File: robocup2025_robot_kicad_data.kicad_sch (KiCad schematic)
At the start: 3 parts, among them U2 ESP32-DEVKITC-32E, U4 RASPBERRY_PI_4B_4GB

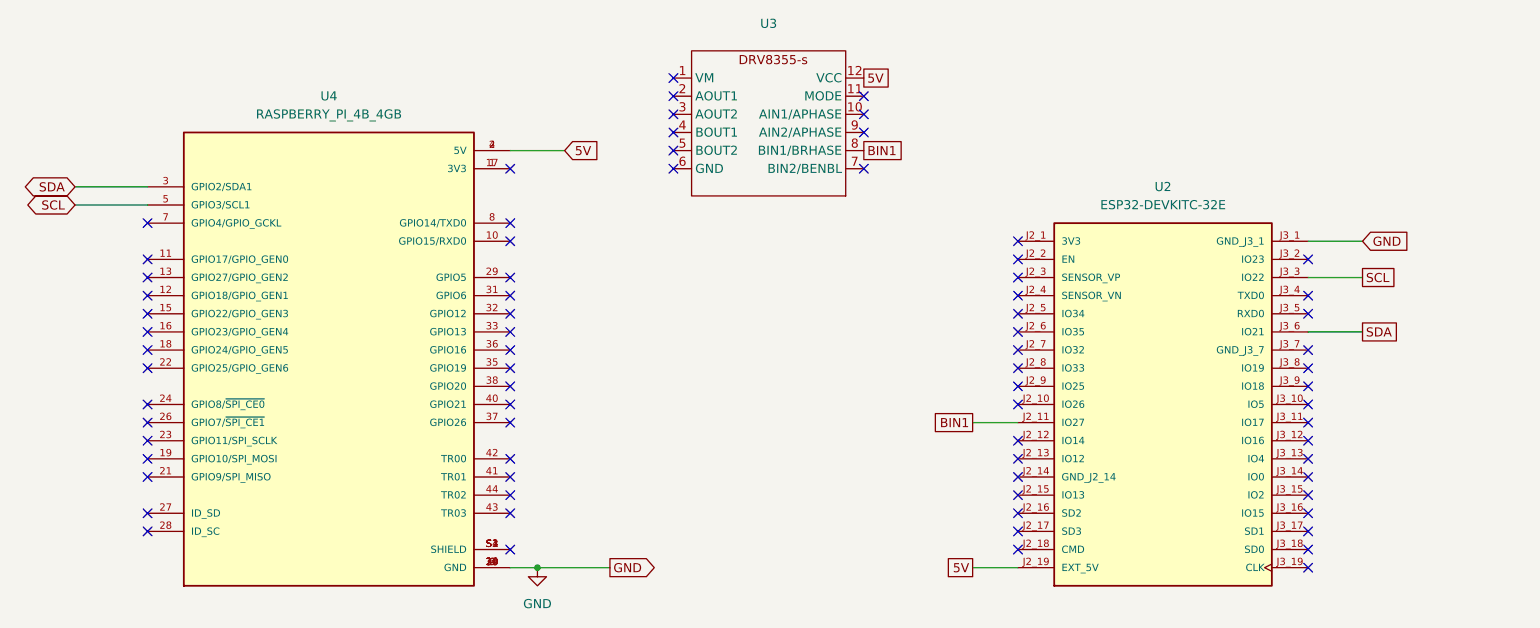
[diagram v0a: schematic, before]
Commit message: made sch
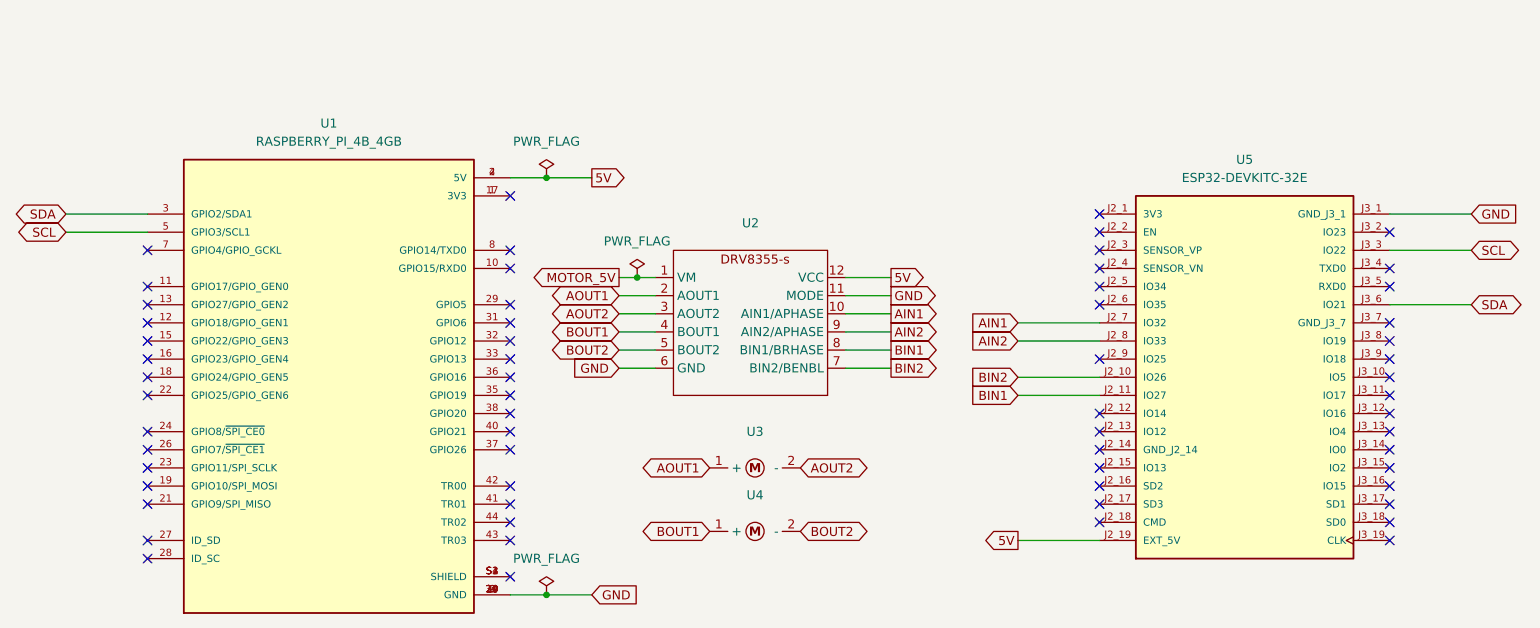
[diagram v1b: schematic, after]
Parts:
- removed U2: ESP32-DEVKITC-32E, ESP32-DEVKITC-32E:MODULE_ESP32-DEVKITC-32E, symbol robo:ESP32-DEVKITC-32E
- removed U3: ~, symbol robo:DRV8835-s
- removed U4: RASPBERRY_PI_4B_4GB, RASPBERRY_PI_4B_4GB:MODULE_RASPBERRY_PI_4B_4GB, symbol robo:RASPBERRY_PI_4B_4GB
- added U1: RASPBERRY_PI_4B_4GB, RASPBERRY_PI_4B_4GB:MODULE_RASPBERRY_PI_4B_4GB, symbol robo:RASPBERRY_PI_4B_4GB
- added U2: ~, symbol robo:DRV8835-s
- added U3, U4: ~, symbol robo:DC_MOTOR
- added U5: ESP32-DEVKITC-32E, ESP32-DEVKITC-32E:MODULE_ESP32-DEVKITC-32E, symbol robo:ESP32-DEVKITC-32E
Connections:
- net 5V: now also U1.2 (5V), U1.4 (5V), U2.12 (VCC), U5.J2_19 (EXT_5V)
- net BIN1: now also U2.8 (BIN1/BRHASE), U5.J2_11 (IO27)
- net GND: now also U1.14 (GND), U1.20 (GND), U1.25 (GND), U1.30 (GND), U1.34 (GND), U1.39 (GND), U1.6 (GND), U1.9 (GND), U2.11 (MODE), U2.6 (GND), U5.J3_1 (GND_J3_1)
- net SCL: now also U1.5 (GPIO3/SCL1), U5.J3_3 (IO22)
- net SDA: now also U1.3 (GPIO2/SDA1), U5.J3_6 (IO21)
- new net: U1.1 (3V3), U1.17 (3V3)
- new net: U1.S1 (SHIELD), U1.S2 (SHIELD), U1.S3 (SHIELD), U1.S4 (SHIELD)
- new net AIN1: U2.10 (AIN1/APHASE), U5.J2_7 (IO32)
- new net AIN2: U2.9 (AIN2/APHASE), U5.J2_8 (IO33)
- new net AOUT1: U2.2 (AOUT1), U3.1 (+)
- new net AOUT2: U2.3 (AOUT2), U3.2 (-)
- new net BIN2: U2.7 (BIN2/BENBL), U5.J2_10 (IO26)
- new net BOUT1: U2.4 (BOUT1), U4.1 (+)
- new net BOUT2: U2.5 (BOUT2), U4.2 (-)
- new net MOTOR_5V: U2.1 (VM)
- no-connect marks 75 -> 62
